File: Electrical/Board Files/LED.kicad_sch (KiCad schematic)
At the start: 14 parts

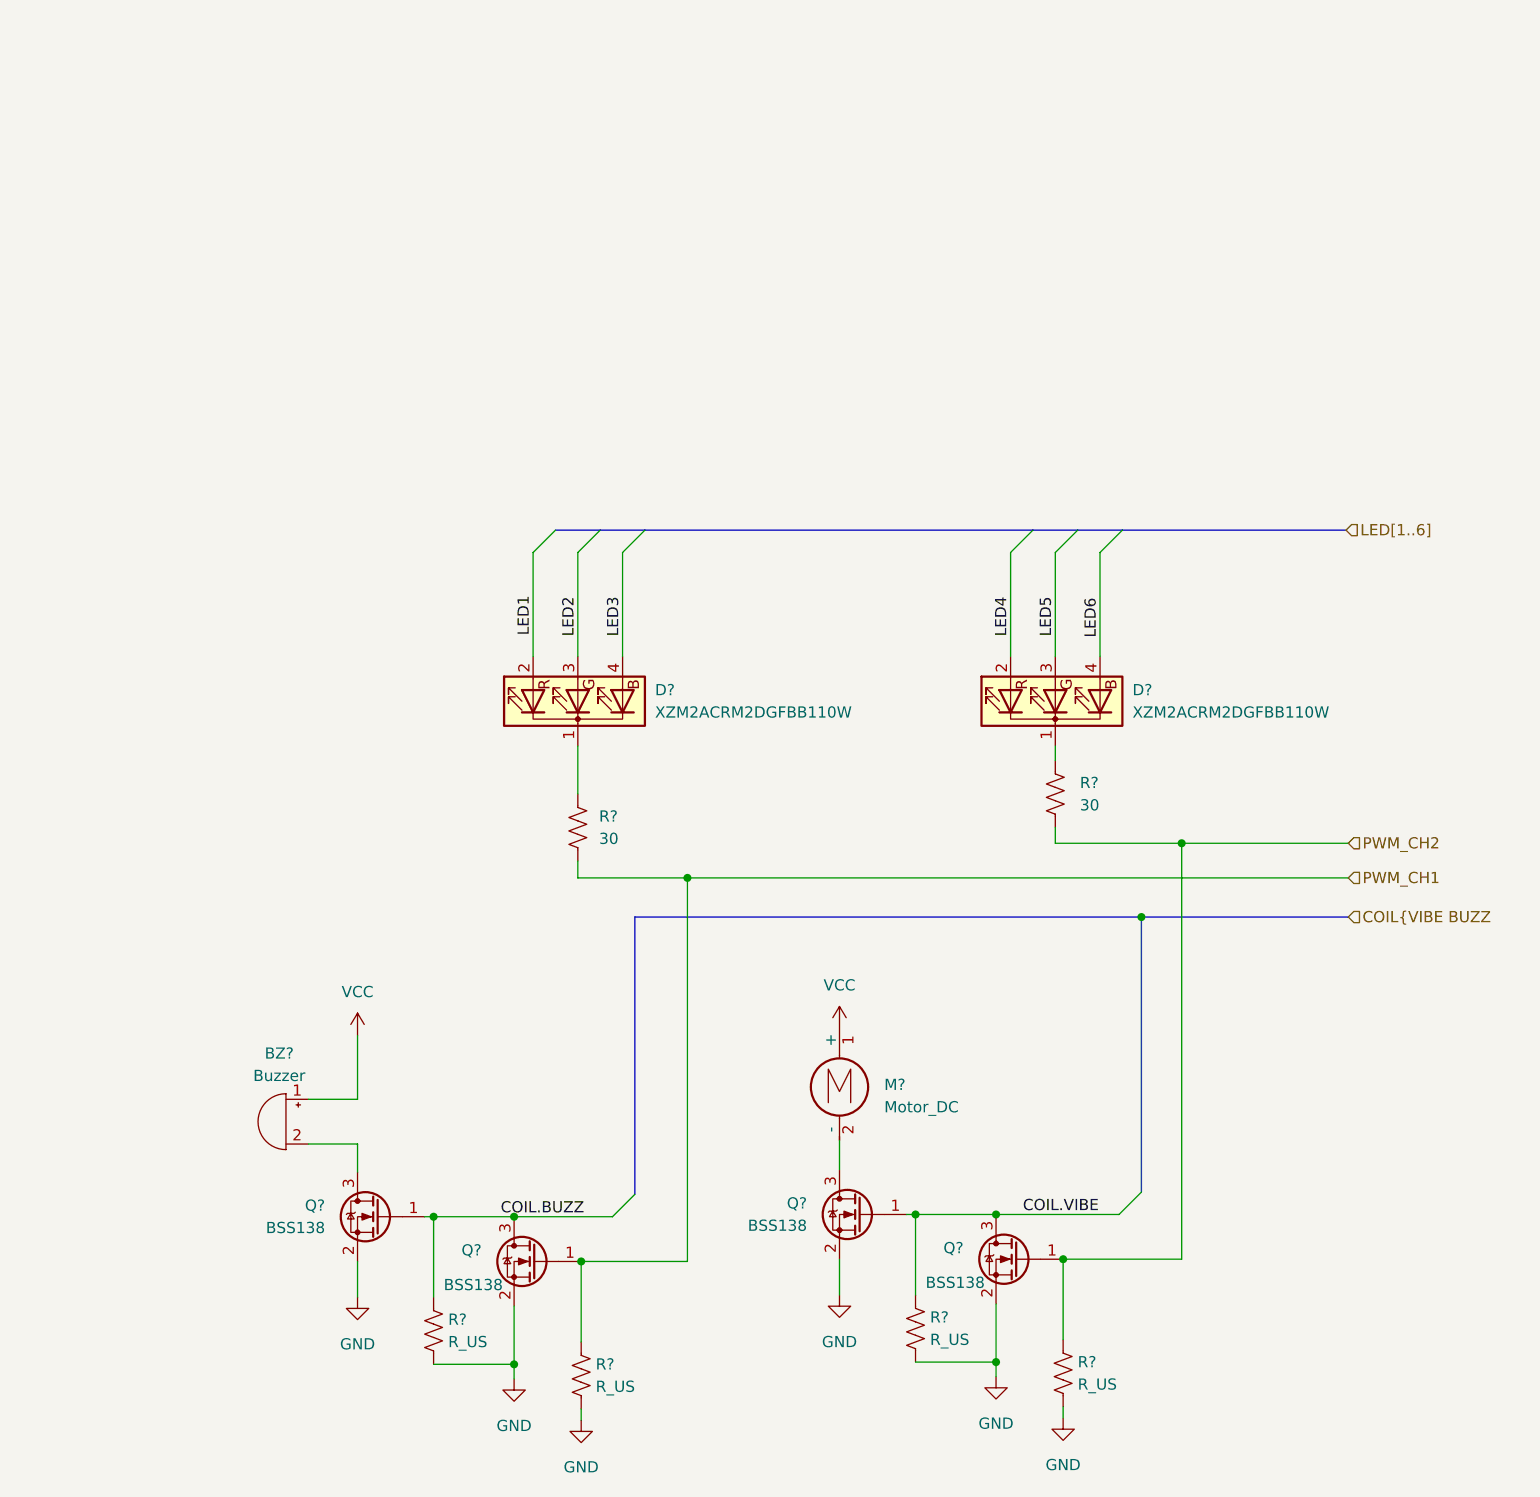
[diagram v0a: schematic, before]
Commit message: Added Xbee libs and bus aliases
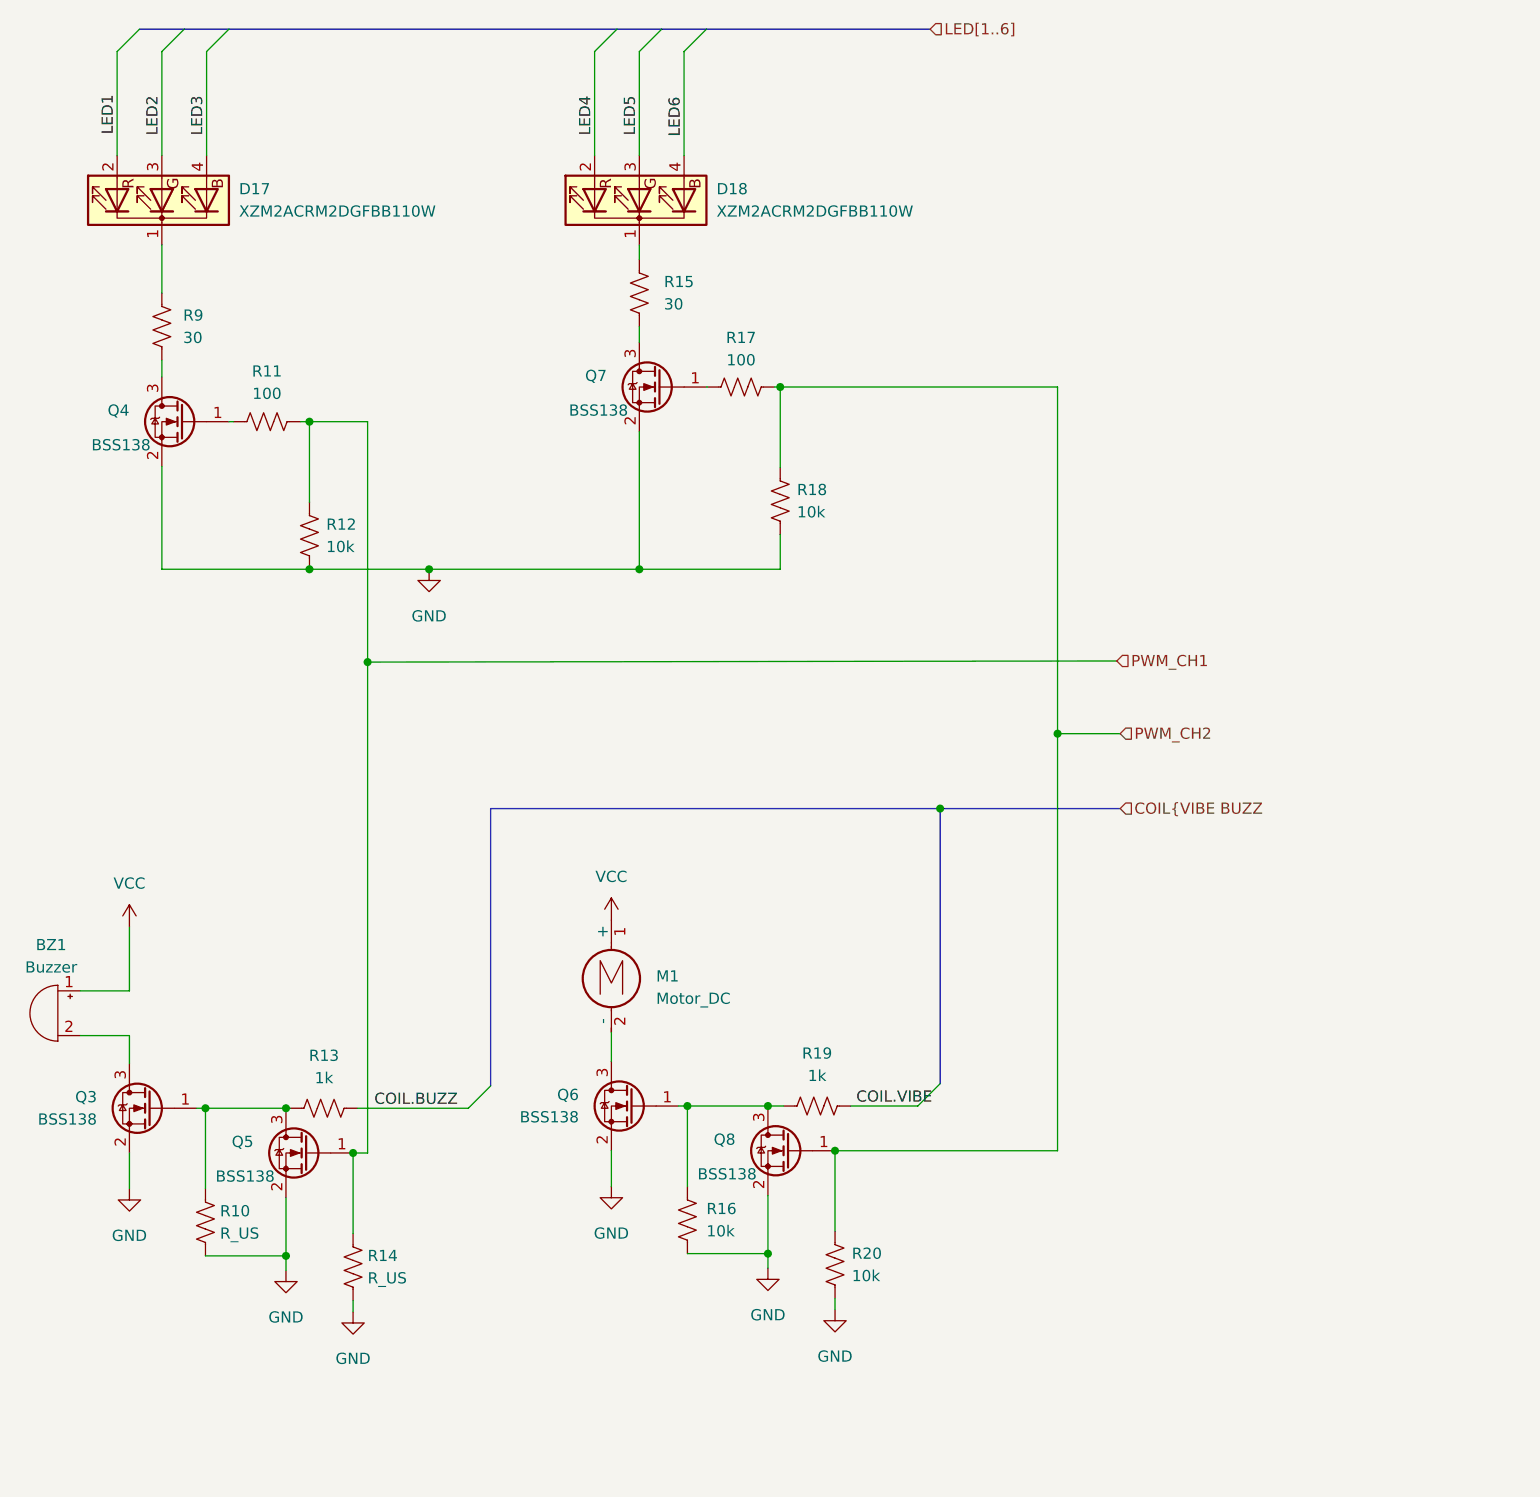
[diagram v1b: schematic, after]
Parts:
- added Q4, Q7: BSS138, Package_TO_SOT_SMD:SOT-23, symbol Transistor_FET:BSS138
- added R11, R17: 100, symbol Device:R_US
- added R12, R18: 10k, symbol Device:R_US
- added R13, R19: 1k, symbol Device:R_US
- R16, R20: renamed from R?; value R_US -> 10k
- gave numbers to parts that had none: 12
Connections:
- net COIL.BUZZ: now also R13.2; no longer Q3.1 (G), Q5.3 (D), R10.1
- net COIL.VIBE: now also R19.2; no longer Q6.1 (G), Q8.3 (D), R16.1
- net GND: now also Q4.2 (S), Q7.2 (S), R12.2, R18.2
- net PWM_CH1: now also R11.2, R12.1; no longer R9.2
- net PWM_CH2: now also R17.2, R18.1; no longer R15.2
- new net: Q7.1 (G), R17.1
- new net: Q7.3 (D), R15.2
- new net: Q3.1 (G), Q5.3 (D), R10.1, R13.1
- new net: Q6.1 (G), Q8.3 (D), R16.1, R19.1
- new net: Q4.3 (D), R9.2
- new net: Q4.1 (G), R11.1
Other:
- title: (none) -> Robotics Controller
- moved on the sheet: BZ1, D17, D18, M1, Q3, Q5, Q6, Q8, R10, R14, R15, R16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

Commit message: Updating title block fields and adding pdf schematic
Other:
- company: (none) -> Rockerbotics
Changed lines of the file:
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@@
   (title_block
     (title "Robotics Controller")
+    (date "2022-09-02")
     (rev "A")
+    (company "Rockerbotics")
   )
   (junction (at 55.626 146.304) (diameter 0) (color 0 0 0 0)
